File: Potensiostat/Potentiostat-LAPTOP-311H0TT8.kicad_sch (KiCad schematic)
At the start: 0 parts

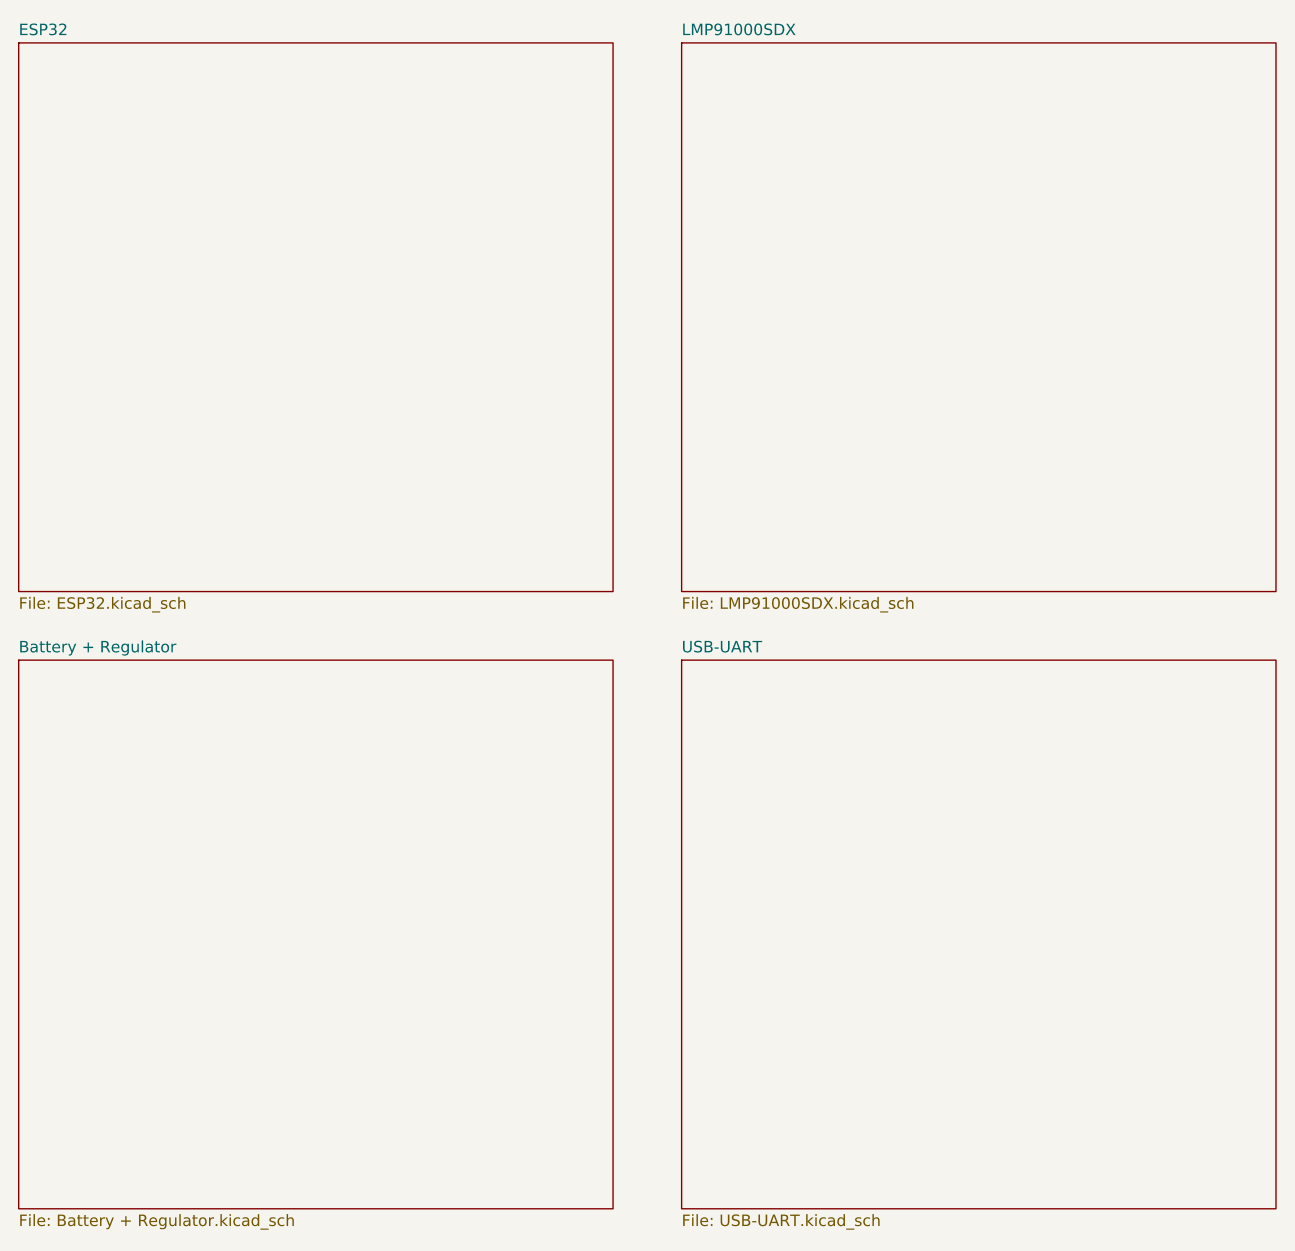
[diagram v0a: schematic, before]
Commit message: LMP USB Update
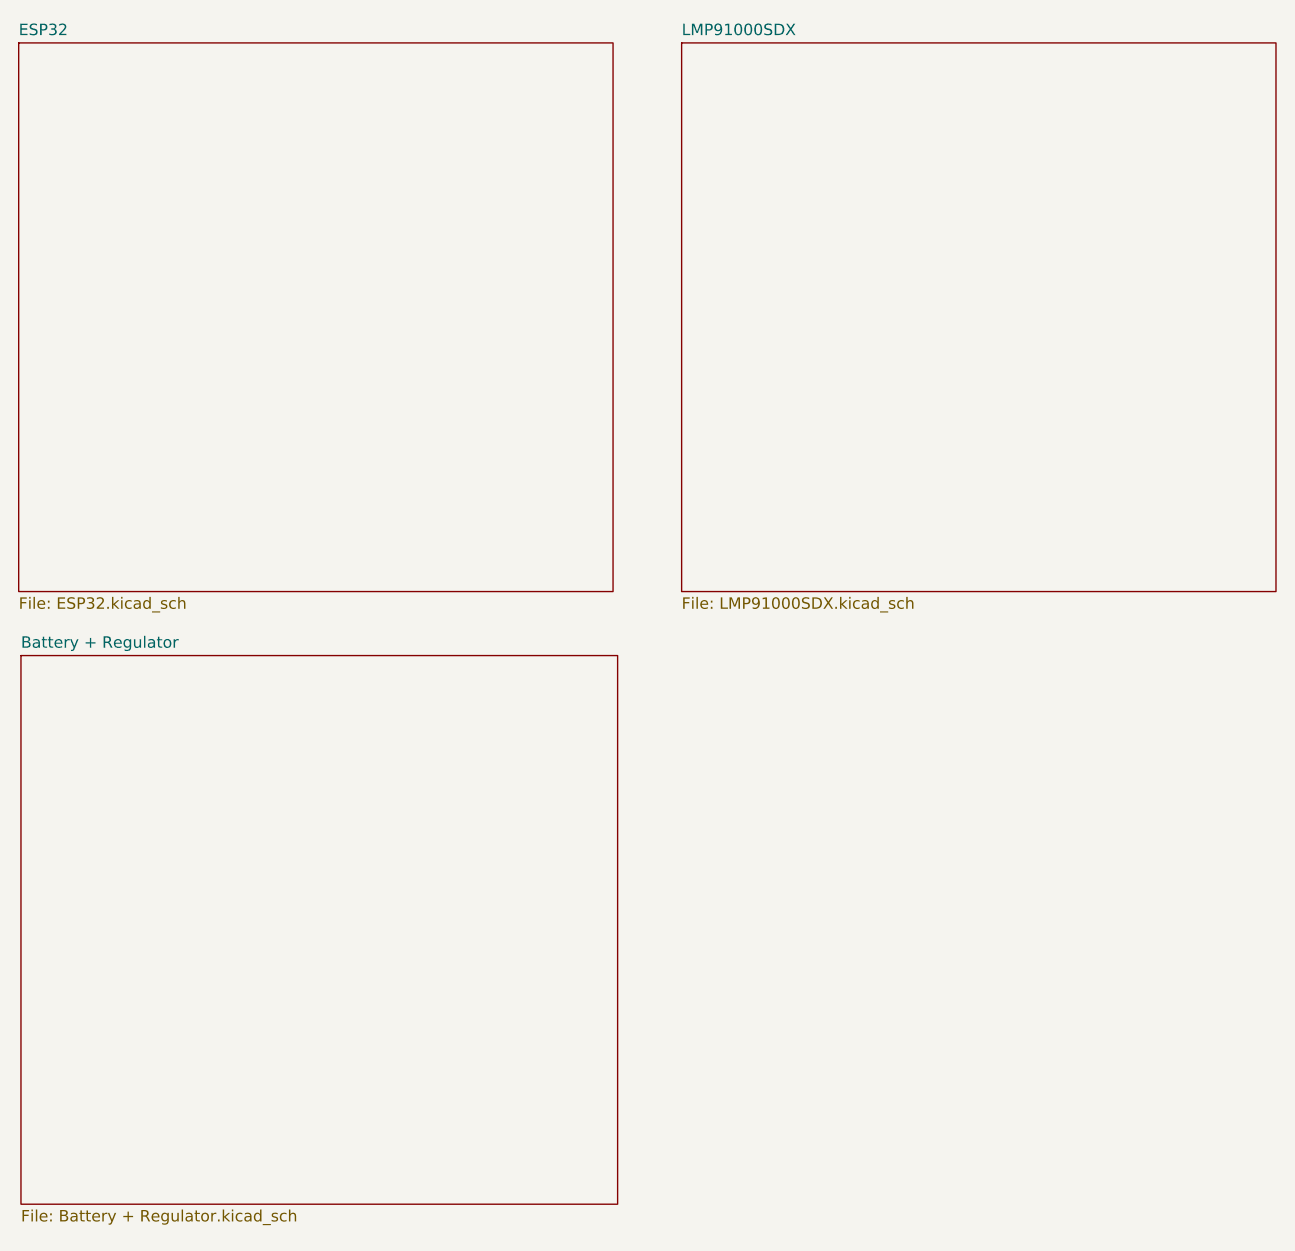
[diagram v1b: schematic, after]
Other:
- removed sheet USB-UART
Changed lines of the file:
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@@
-	)
-	(sheet
-		(at 91.44 87.63)
-		(size 66.04 60.96)
-		(exclude_from_sim no)
-		(in_bom yes)
-		(on_board yes)
-		(dnp no)
-		(fields_autoplaced yes)
-		(stroke
-			(width 0.1524)
-			(type solid)
-		)
-		(fill
-			(color 0 0 0 0.0000)
-		)
-		(property "Sheetname" "USB-UART"
-			(at 91.44 86.9184 0)
-			(effects
-				(font
-					(size 1.27 1.27)
-				)
-				(justify left bottom)
-			)
-		)
-		(property "Sheetfile" "USB-UART.kicad_sch"
-			(at 91.44 149.1746 0)
-			(effects
-				(font
-					(size 1.27 1.27)
-				)
-				(justify left top)
-			)
-		)
-		(instances
-			(project "Potentiostat"
-				(path "/be108998-ac86-4f7d-931a-841db1905f2a"
-					(page "5")
-				)
-			)
-		)
 	)
 	(sheet
@@
 	)
 	(sheet
-		(at 17.78 87.63)
-		(size 66.04 60.96)
+		(at 18.034 87.122)
+		(size 66.294 60.96)
 		(exclude_from_sim no)
 		(in_bom yes)
@@
 		)
 		(property "Sheetname" "Battery + Regulator"
-			(at 17.78 86.9184 0)
+			(at 18.034 86.4104 0)
 			(effects
 				(font
@@
 		)
 		(property "Sheetfile" "Battery + Regulator.kicad_sch"
-			(at 17.78 149.1746 0)
+			(at 18.034 148.6666 0)
 			(effects
 				(font
